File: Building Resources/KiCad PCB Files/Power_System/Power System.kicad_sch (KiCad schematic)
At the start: 15 parts, among them J1 Conn_01x02_Socket, J2 Conn_01x02_Socket, J3 Conn_01x02_Socket, J4 Conn_01x02_Socket, J5 Conn_01x02_Socket, U1 LM2596T-3.3

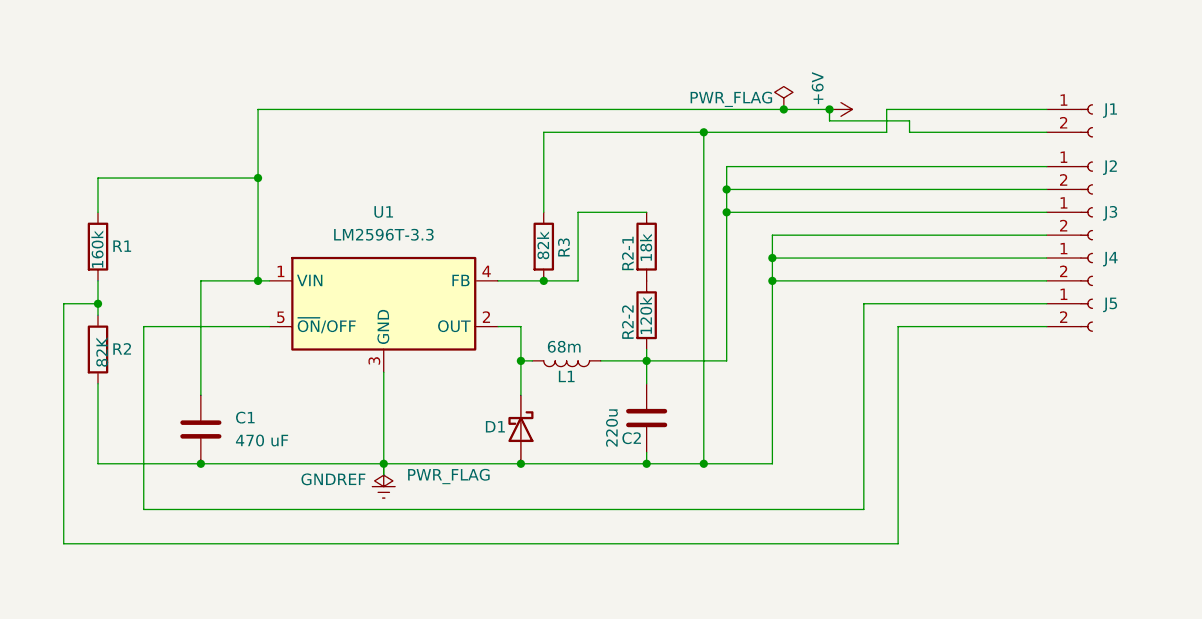
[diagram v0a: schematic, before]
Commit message: Update KiCad Files (#59)
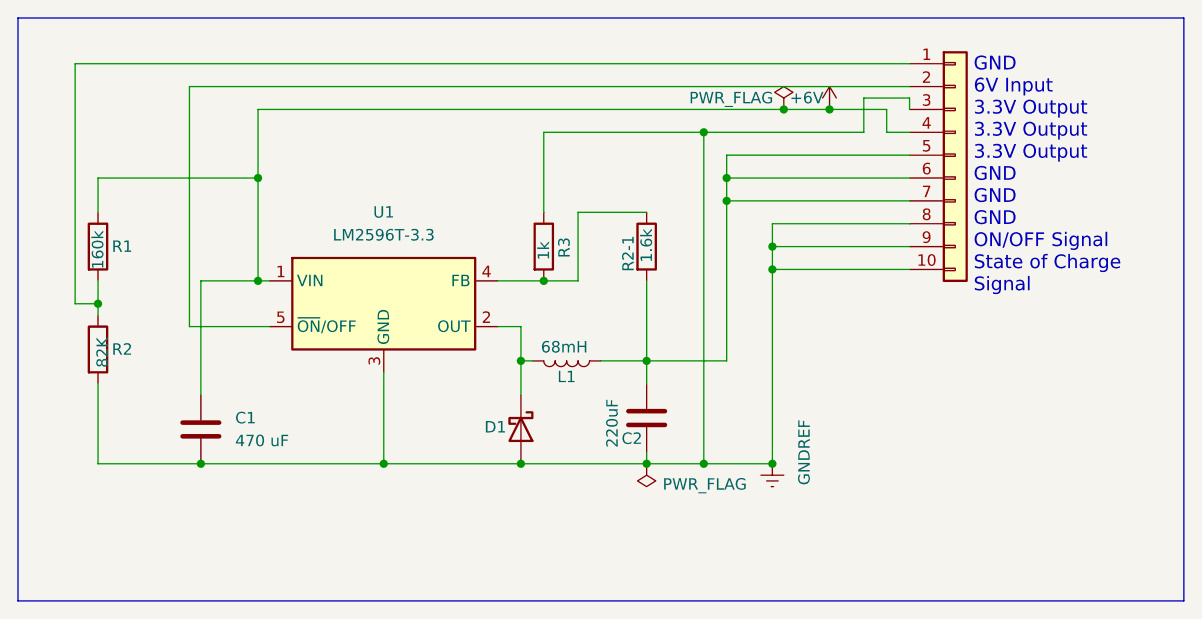
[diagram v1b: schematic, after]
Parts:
- removed J1, J2, J3, J4, J5: Conn_01x02_Socket, Connector_PinSocket_2.54mm:PinSocket_1x02_P2.54mm_Vertical, symbol Connector:Conn_01x02_Socket
- removed R2-2: 120k, Resistor_THT:R_Axial_DIN0207_L6.3mm_D2.5mm_P7.62mm_Horizontal, symbol Device:R
- added J1: Conn_01x10, Connector_PinSocket_2.54mm:PinSocket_1x10_P2.54mm_Vertical, symbol Connector_Generic:Conn_01x10
- C2: value 220u -> 220uF
- L1: value 68m -> 68mH
- R2-1: value 18k -> 1.6k
- R3: value 82k -> 1k
- U1: footprint Package_TO_SOT_THT:TO-220-5_P3.4x3.7mm_StaggerOdd_Lead3.8mm_Vertical -> LM2596TVADJG:TO170P470X1016X2092-5P
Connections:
- net +6V: now also J1.4 (Pin_4)
- net GNDREF: now also J1.10 (Pin_10), J1.3 (Pin_3), J1.8 (Pin_8), J1.9 (Pin_9)
- net at R1.2, R2.1: now also J1.1 (Pin_1)
- net at R2-1.2: now also C2.1, L1.1, J1.5 (Pin_5), J1.6 (Pin_6), J1.7 (Pin_7)
- net at U1.5 (~{ON}/OFF): now also J1.2 (Pin_2)
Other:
- note added: "GND 6V Input 3.3V Output 3.3V Output 3.3V Output GND GND GND ON/OFF Signal State of Charge Signal"
